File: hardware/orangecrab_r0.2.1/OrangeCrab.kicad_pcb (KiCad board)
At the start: 6 copper layers, 50.8 x 22.9 mm, 163 parts, among them J1 Conn_01x12_Male, J2 Conn_01x16_Male, J3 USB_C_Receptacle_USB2.0, J4 MicroSd, J5 JST, J6 Conn_01x05_Male, SW1 SW_Push, U1 TLV62569DRL, U10 NCP115-2.5, U2 TLV62569DRL, U3 LFE5U-25F-8MG285C, U4 MT41K64M16TW-107_J-TR, U5 BQ24232, U6 W25Q128JVP, U7 TLV62569DRL, U9 74HC4067BQ

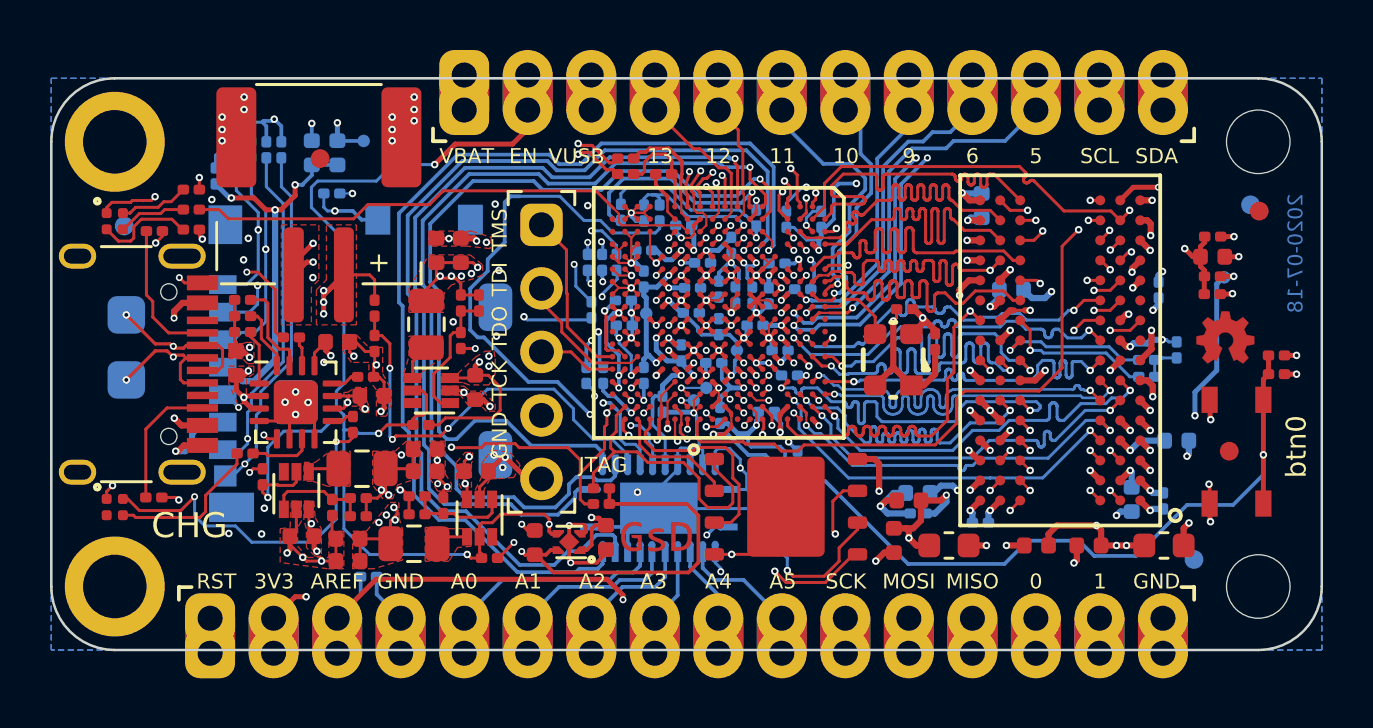
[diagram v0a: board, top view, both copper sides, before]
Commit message: refresh
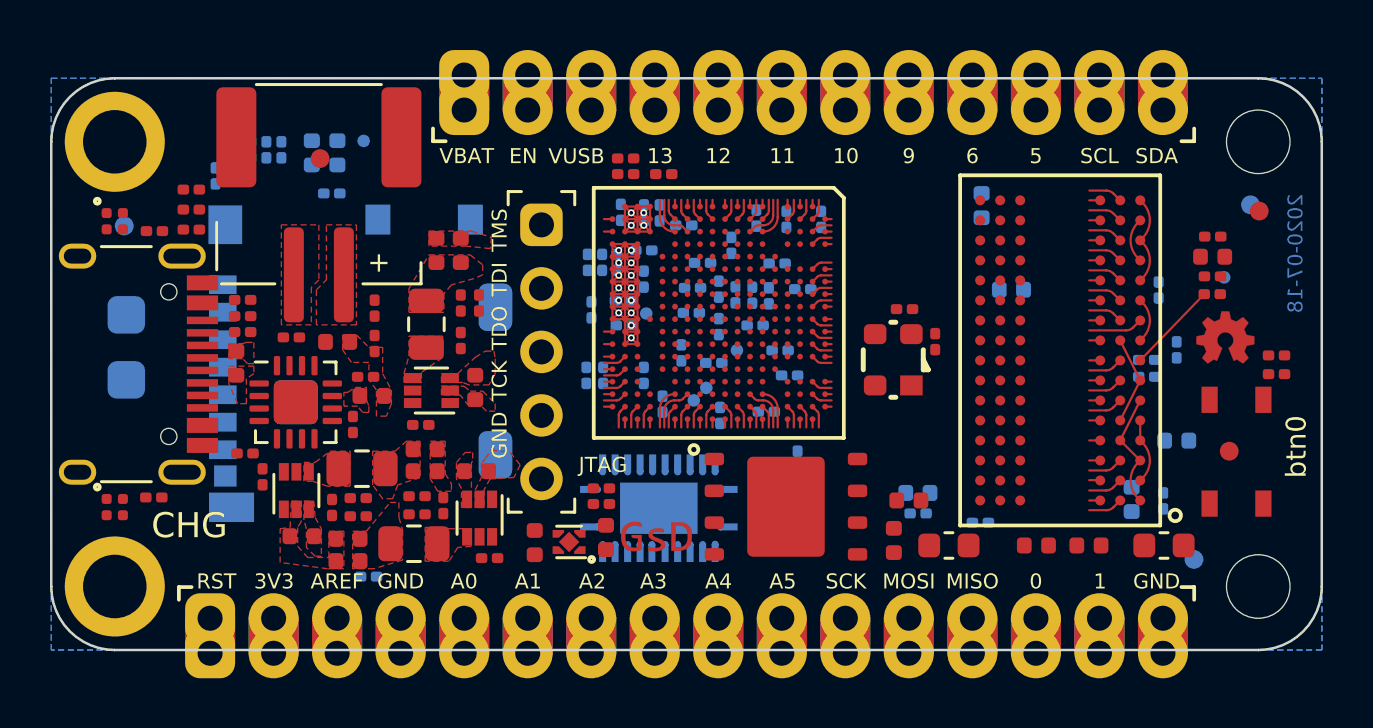
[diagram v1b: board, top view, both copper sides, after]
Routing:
- net GND: track 250.6 -> 67.2 mm, vias 141 -> 18
- net P1.35V: track 102.9 -> 2.18 mm, vias 20 -> 0
- net P3.3V: track 86.1 -> 0.00 mm, vias 20 -> 0
- net P1.1V: track 58.4 -> 0.00 mm, vias 16 -> 0
- net EN: track 49.2 -> 0.00 mm, vias 5 -> 0
- net ECP5_VREF: track 52.6 -> 4.54 mm, vias 8 -> 0
- net VSYS: track 44.2 -> 0.00 mm, vias 13 -> 0
- net SD0_DAT0: track 41.7 -> 0.27 mm, vias 2 -> 0
- net ADC_MUX0: track 41.2 -> 0.00 mm, vias 1 -> 0
- net ADC_MUX1: track 42.1 -> 1.60 mm, vias 1 -> 0
- net LED_R: track 40.4 -> 0.00 mm, vias 2 -> 0
- net LED_B: track 39.4 -> 0.00 mm, vias 2 -> 0
- net SD0_DAT1: track 38.6 -> 0.00 mm, vias 2 -> 0
- net ADC_CTRL1: track 35.6 -> 0.27 mm, vias 1 -> 0
- net ADC_MUX3: track 34.5 -> 0.27 mm, vias 1 -> 0
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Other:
- net class DDR3_CTRL_LM1.0 removed
- net class DDR3_DQS0_LM1.0 removed
- net class DDR3_DQS1_LM1.0 removed
- net class DDR_CLK_LM1.0 removed
- net class Default removed
